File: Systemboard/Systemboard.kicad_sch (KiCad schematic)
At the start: 7 parts, among them J1 Conn_01x60, J108 Prog BT, U101 ESP32-WROOM-32E

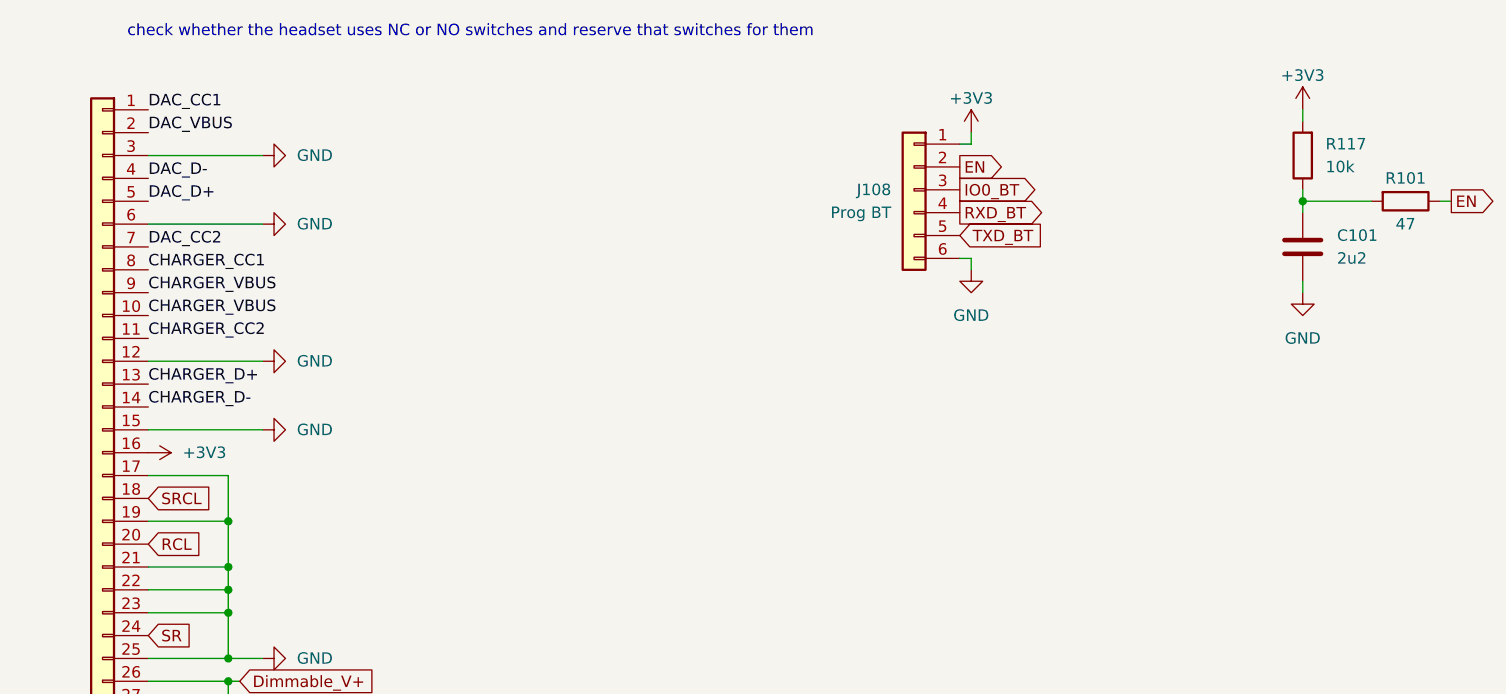
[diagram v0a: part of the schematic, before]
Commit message: Update Systemboard.kicad_sch
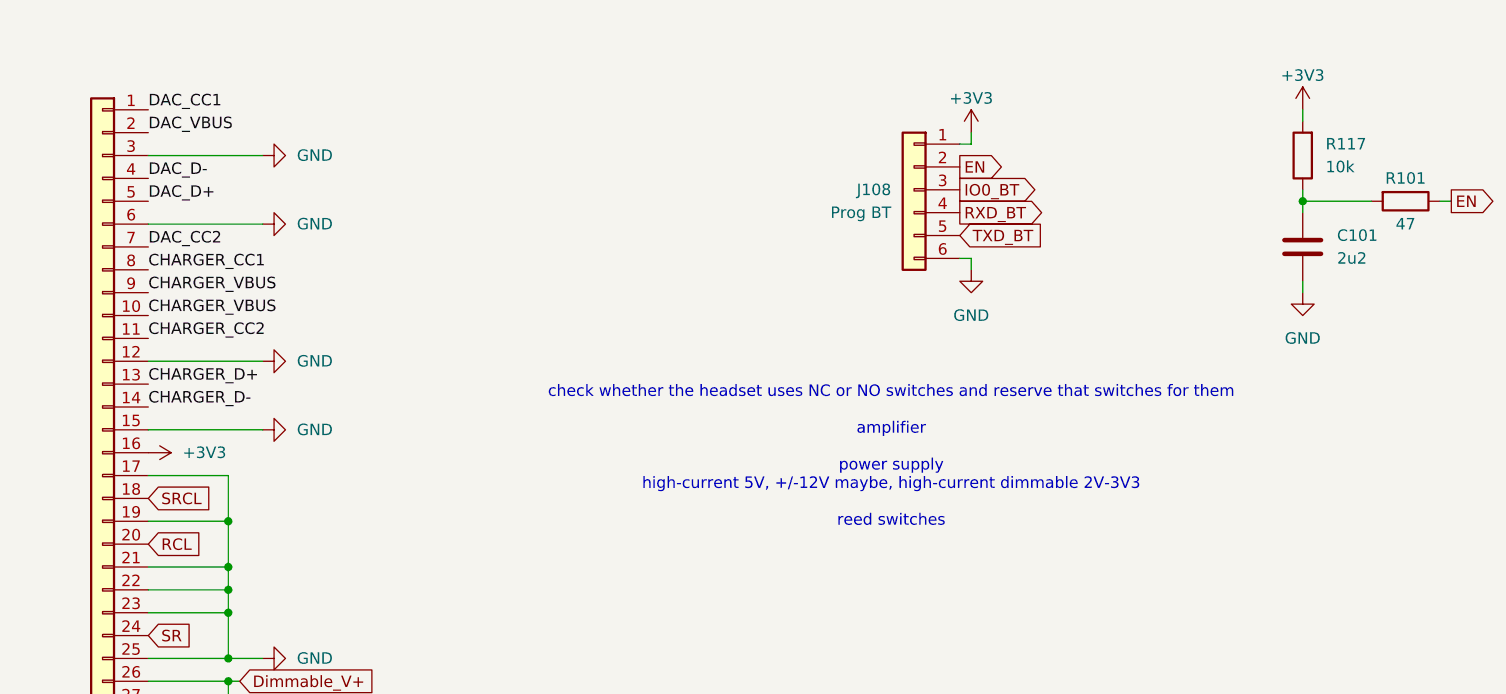
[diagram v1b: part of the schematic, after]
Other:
- note added: "check whether the headset uses NC or NO switches and reserve that switches for them amplifier power supply high-current 5V, +/-12V maybe, high-current dimmable 2V-3V3 reed switches"
- note removed: "check whether the headset uses NC or NO switches and reserve that switches for them"
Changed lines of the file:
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@@
 	(generator_version "9.0")
 	(paper "A4")
-	(text "check whether the headset uses NC or NO switches and reserve that switches for them"
+	(text "check whether the headset uses NC or NO switches and reserve that switches for them\n\namplifier\n\npower supply\nhigh-current 5V, +/-12V maybe, high-current dimmable 2V-3V3\n\nreed switches"
 		(exclude_from_sim no)
-		(at 67.564 18.034 0)
+		(at 114.3 65.278 0)
 		(effects
 			(font
